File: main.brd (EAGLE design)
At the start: 130 x 65 mm, 302 parts, among them CN1 DC-012A-D010, CN2 JST GH 10 Pin, CN3 5.8ZSPT, CN4 8 PIN FFC, CN5 MC-118LS-H100, CN7 8 PIN FFC, Q1 GSFP0449, Q2 2SCR586D, Q3 MMBT3904, Q4 MMBT3906, Q5 MMBT3906, U1 TPS54302, U10 SN74LVC2G17, U11 SN74LVC2G17, U12 SN74LVC2G17, U13 SN74LVC2G17, U14 SN74LVC2G17, U15 SN74LVC2G17, U16 SN74LVC2G17, U17 SN74LVC2G17, U18 T8Q144C4, U19 SN74LVC2G17, U2 USBLC6-2SC6, U20 R2A20169SA#W5, U21 LM317MDT, U22 LM317MDT, U23 ADC101C027, U27 ADS7056, U28 AD5258BRMZ1-R7, U29 COS8092SR, U3 93LC56B-I/SN, U30 ADS7056, U31 AD5258BRMZ1-R7, U32 COS8092SR, U33 LM317MDT, U34 LM317MDT, U35 ADS7056, U36 AD5258BRMZ1-R7, U37 COS8092SR, U4 W25Q128JV, U41 ADS7056, U42 AD5258BRMZ1-R7, U43 COS8092SR, U44 ADS7056, U45 AD5258BRMZ1-R7, U46 COS8092SR, U5 TPS62065, U50 ADS7056, U51 AD5258BRMZ1-R7, U52 COS8092SR, U6 FT2232H, U7 TPS563201, U8 TCD2720BFG, U9 SN74LVC2G17

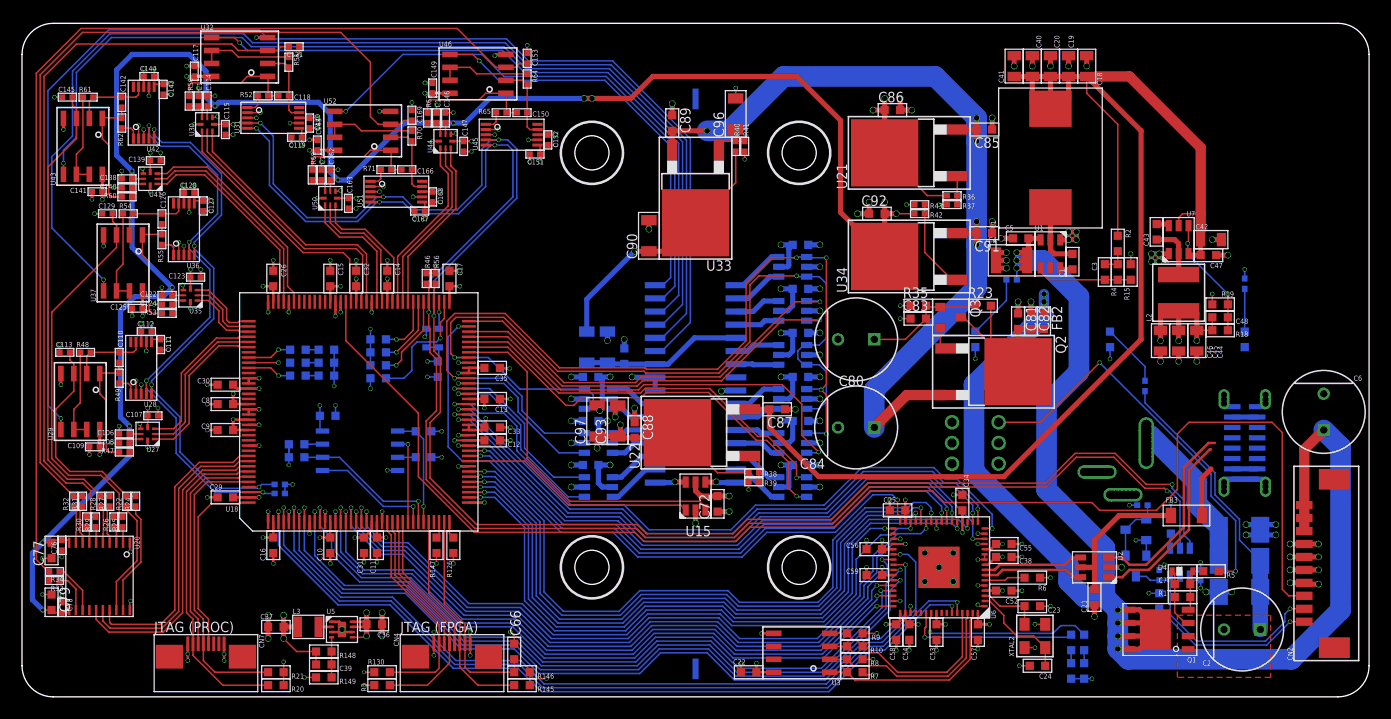
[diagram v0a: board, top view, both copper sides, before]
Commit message: Bits and pieces
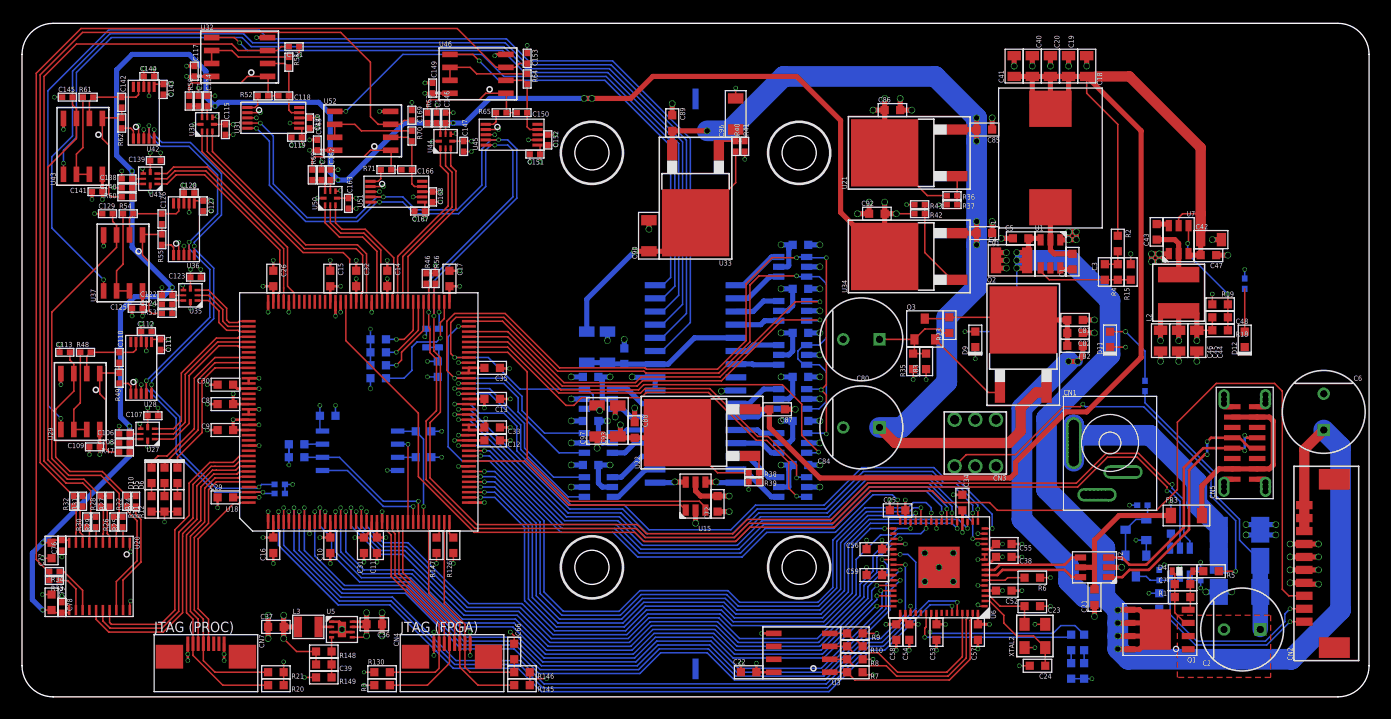
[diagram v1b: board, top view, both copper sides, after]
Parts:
- moved R59 22.5 mm to (-52.5, -13.9), flipped to the top, turned to 270 degrees
- moved R11 20.7 mm to (-51.2, -13.9), flipped to the top, turned to 270 degrees
- moved R12 19.0 mm to (-50.0, -13.9), flipped to the top, turned to 270 degrees
- moved D10 18.6 mm to (-52.5, -11.1), flipped to the top, turned to 270 degrees
- moved D5 16.9 mm to (-51.2, -11.1), flipped to the top, turned to 270 degrees
- moved D6 15.1 mm to (-50.0, -11.1), flipped to the top, turned to 270 degrees
- moved C81 5.50 mm to (36.6, 3.88), turned to 180 degrees
- moved R35 5.40 mm to (21.0, -0.12), turned to 90 degrees
- moved R58 4.53 mm to (31.0, 3.25), turned to 90 degrees
- moved C82 4.40 mm to (36.6, 2.62), turned to 180 degrees
- moved C83 4.19 mm to (22.2, -0.12), turned to 90 degrees
- moved Q2 3.95 mm to (31.6, 2.12), turned to 0 degrees
- moved FB2 3.83 mm to (36.6, 1.38), turned to 180 degrees
- moved R23 3.75 mm to (24.5, 3.38), turned to 90 degrees
- moved Q3 2.74 mm to (22.1, 3.00), turned to 0 degrees
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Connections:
- removed net PROC_STATUS: U18.117
- net LED_PROC_STATUS: now also U18.117
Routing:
- net LED_PROC_STATUS: track 0.00 -> 15.4 mm
- net PWR_ANA_UNREG: track 85.5 -> 98.4 mm
- net LED_PROC_SCANNING: track 4.31 -> 16.9 mm, vias 1 -> 0
- net N$5: track 14.9 -> 26.1 mm
- net LED_FPGA_STATUS: track 4.31 -> 14.4 mm, vias 1 -> 0
- net N$41: track 9.66 -> 18.9 mm
- net LED_PWM_CONT: track 133.1 -> 139.2 mm
- net N$13: track 18.4 -> 24.4 mm, vias 0 -> 2
- net N$40: track 2.43 -> 8.37 mm
- net N$12: track 18.8 -> 24.3 mm, vias 0 -> 2
- net PROC_STATUS: track 2.88 -> 0.00 mm, vias 1 -> 0
- net N$11: track 39.3 -> 42.0 mm
- net GND: track 251.0 -> 253.4 mm
- net N$39: track 11.9 -> 10.00 mm
- net PWR_SYS_12V: track 138.8 -> 140.5 mm
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
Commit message: New LED PCB formfactor. UART debug added to FPGA for softcore.
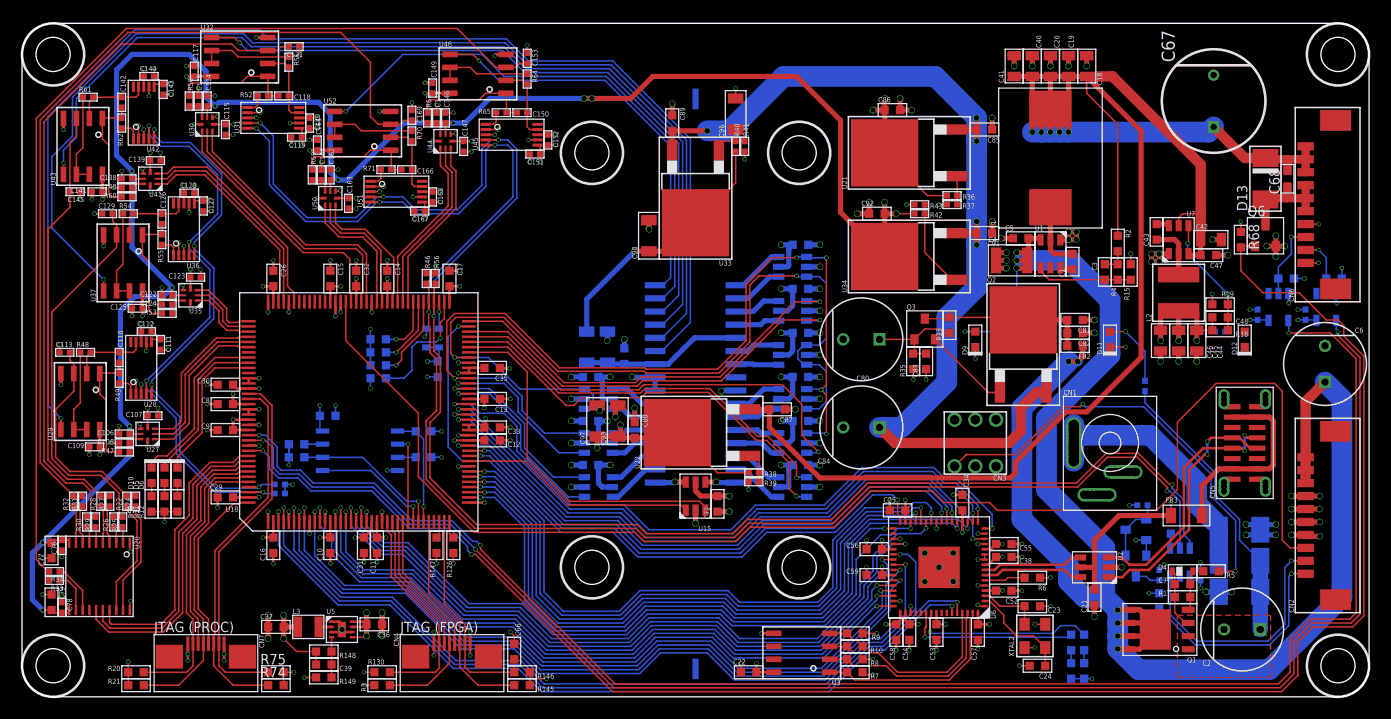
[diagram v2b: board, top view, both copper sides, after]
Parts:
- added C67: 470uF 25V, CAPACITORS:10MM_RADIAL_5MM_PITCH
- added C68: 0.1uF 50V, c_0603:0603
- added C69, C70: 0.1uF 16V, c_0402:0402
- added CN6: JST GH 10 Pin, CONNECTORs:1.25-10PWT
- added D13: B360A-13-F, DIODES:DO214AC
- added MECH5, MECH6, MECH7, MECH8: 6mm x 3mm, MISC:MOUNTHOLE_6X3
- added Q6: IRLML6244, TRANSISTORs:SOT23-3
- added R68, R72, R73, R74, R75: 10k, r_0603:0603
- added U24, U25: SCHMITT, ICs:SOT23-5
- moved R20 13.6 mm to (-54.0, -30.1), turned to 180 degrees
- moved R21 13.6 mm to (-54.0, -31.4), turned to 180 degrees
- moved C145 9.16 mm to (-59.9, 16.2), turned to 180 degrees
- moved R67 5.20 mm to (50.6, 2.75), turned to 0 degrees
- moved C6 4.63 mm to (60.8, -0.38)
- moved CN2 4.63 mm to (61.0, -15.0)
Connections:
- removed net N$76: U18.134
- removed net N$77: U18.132
- removed net N$78: U18.131
- removed net N$79: U18.124
- removed net N$80: U18.123
- new net MTR_PWM: Q6.1, R68.2, U18.134
- new net MTR_SENSE_A: U18.131, U24.4
- new net MTR_SENSE_B: U18.132, U25.4
- new net MTR_SENSE_IN_A: CN6.3, R72.2, U24.2
- new net MTR_SENSE_IN_B: CN6.2, R73.2, U25.2
- new net N$57: C68.1, CN6.5, CN6.6, CN6.7, D13.A, Q6.2
- new net PROC_UART_RX: CN7.2, R75.1, U18.123
- new net PROC_UART_TX: CN7.3, R74.1, U18.124
- net GND: now also C67.1, C69.1, C70.1, CN6.1, Q6.3, R68.1, R72.1, R73.1, U24.3, U25.3
- net PWR_SYS_12V: now also C67.2, C68.2, CN6.10, CN6.8, CN6.9, D13.K
- net PWR_SYS_3V3: now also C69.2, C70.2, CN6.4, R74.2, R75.2, U24.5, U25.5
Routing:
- net MTR_PWM: track 0.00 -> 167.6 mm, vias 0 -> 2
- net MTR_SENSE_A: track 0.00 -> 156.1 mm, vias 0 -> 3
- net MTR_SENSE_B: track 0.00 -> 152.4 mm, vias 0 -> 3
- net PWR_SYS_12V: track 140.5 -> 185.3 mm, vias 0 -> 5
- net PROC_UART_TX: track 0.00 -> 35.4 mm
- net PROC_UART_RX: track 0.00 -> 35.0 mm
- net GND: track 253.4 -> 264.7 mm, vias 251 -> 263
- net N$57: track 0.00 -> 10.3 mm
- net MTR_SENSE_IN_A: track 0.00 -> 7.34 mm, vias 0 -> 1
- net PWR_SYS_3V3: track 134.7 -> 140.9 mm, vias 66 -> 69
- net MTR_SENSE_IN_B: track 0.00 -> 5.76 mm, vias 0 -> 1
- net PWR_BUS_24V_UNREG: track 167.7 -> 172.6 mm
- net TEMP_SEN_B: track 16.4 -> 21.2 mm
- net TEMP_SEN_A: track 23.2 -> 28.0 mm
- net LED_PWM_CONT: track 139.2 -> 134.7 mm
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
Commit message: Cleared errors on PCB
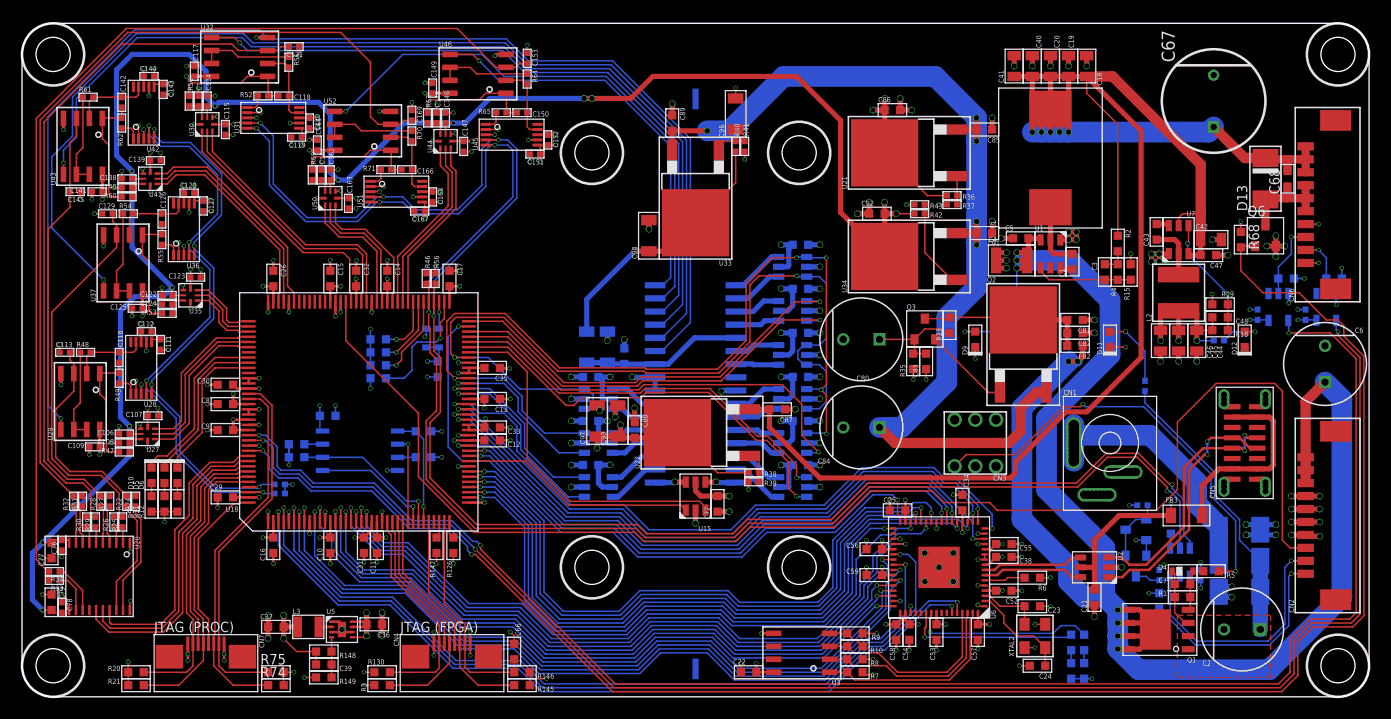
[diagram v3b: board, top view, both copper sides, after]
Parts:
- moved R67 0.88 mm to (50.5, 1.88)
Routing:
- net N$5: track 26.1 -> 31.4 mm
- net N$47: track 0.00 -> 4.36 mm, vias 0 -> 1
- net PWR_SYS_3V3: track 140.9 -> 142.6 mm
- net GND: track 264.7 -> 265.3 mm

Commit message: New formactor
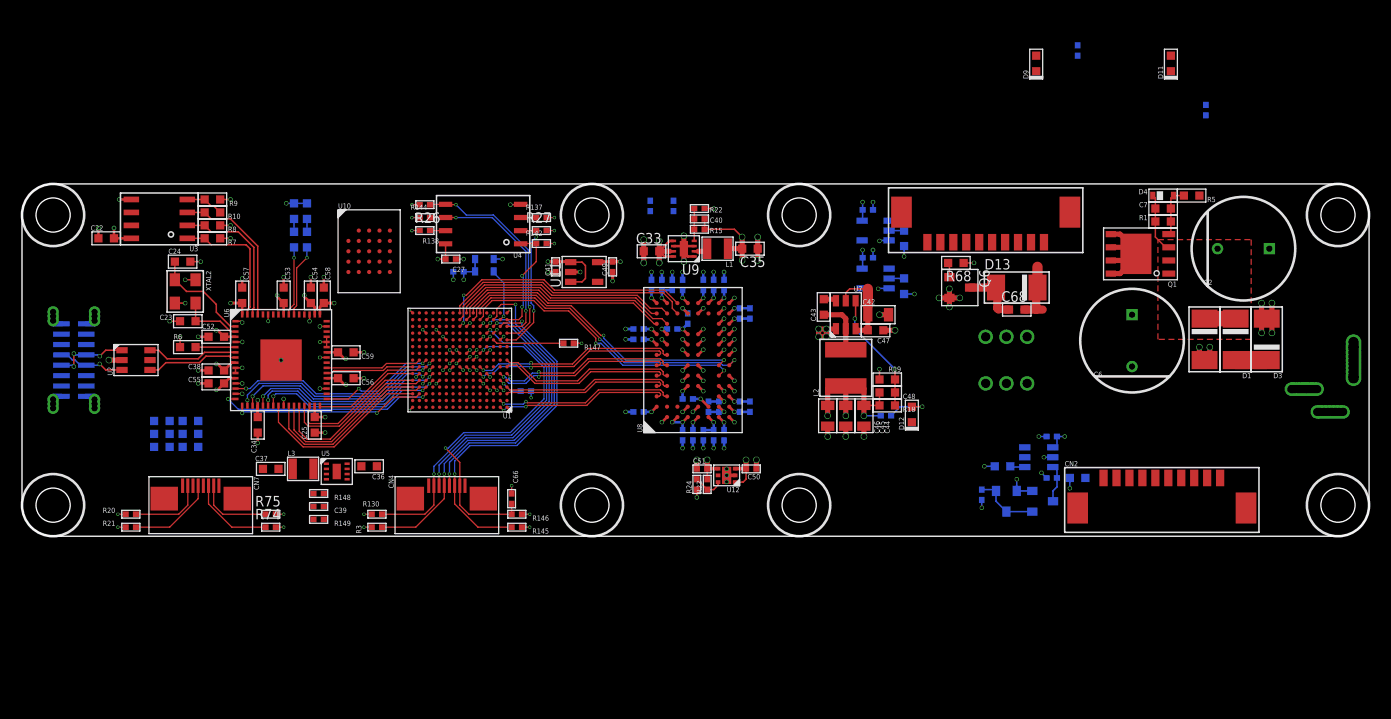
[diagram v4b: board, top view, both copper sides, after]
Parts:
- removed C106, C107, C109, C111, C112, C113, C114, C115, C117, C119, C120, C121, C122, C123, C125, C127, C128, C129, C138, C139, C141, C143, C144, C145, C146, C147, C149, C151, C152, C153, C162, C163, C165, C167, C168, C169, C76, C78: 0.1uF 16V, c_0402:0402
- removed C108, C116, C124, C140, C148, C164: 220pF 25V, c_0402:0402
- removed C110, C118, C126, C142, C150, C166: NO FIT, c_0402:0402
- removed C61, C62, C63, C71, C72, C73, C74, C75: 100nF 16V, CAPACITORS:0603
- removed C67: 470uF 25V, CAPACITORS:10MM_RADIAL_5MM_PITCH
- removed C77, C79: 10uF 10V, c_0603:0603
- removed C80, C84: 100uF 50V, CAPACITORS:8MM_RADIAL_3.5MM_PITCH
- removed C81, C83, C85, C87, C89, C91: 0.1uF 50V, c_0603:0603
- removed C82: 100pF 50V, c_0603:0603
- removed C86, C88, C92: 1uF 10V, c_0603:0603
- removed C90: 1uF 16V, c_1206:1206
- removed C93, C96, C97: 10uF 10V, c_1206:1206
- removed FB1, FB3: 150R 100MHz, INDUCTORS:1206
- removed FB2: 600R, INDUCTORS:0603
- removed Q2: 2SCR586D, TRANSISTORs:TO252
- removed Q3: MMBT3904, TRANSISTORs:SOT23-3
- removed R126, R139, R140, R141: 10k, r_0603:0603
- removed R25, R29, R31, R33: 430R, r_0402:0402
- removed R28, R30, R32, R34: 110k, r_0402:0402
- removed R35: 20k, r_0603:0603
- removed R36, R38, R40, R42: 240R, r_0402:0402
- removed R37, R39: 715R, r_0402:0402
- removed R41: 1.69k, r_0402:0402
- removed R43: 390R, r_0402:0402
- removed R44, R45, R46, R56: 2.2k, r_0402:0402
- removed R47, R50, R53, R60, R63, R69: 100R, r_0402:0402
- removed R48, R51, R54, R61, R64, R70: 330R, r_0402:0402
- removed R49, R52, R55, R62, R65, R71: 680R, r_0402:0402
- removed U13, U14, U15, U16, U17, U19: SN74LVC2G17, ICs:SOT23-6
- removed U18: T8Q144C4, ICs:QFP144
- removed U20: R2A20169SA#W5, ICs:TSSOP20
- removed U21, U22, U33, U34: LM317MDT, ICs:TO252-2
- removed U27, U30, U35, U41, U44, U50: ADS7056, ICs:X2QFN8
- removed U28, U31, U36, U42, U45, U51: AD5258BRMZ1-R7, ICs:MSOP10
- removed U29, U32, U37, U43, U46, U52: COS8092SR, ICs:SO8
- C1, C51: value 100nF 16V -> 1uF 10V; device CAPACITORS:0603 -> c_0402:0402
- C10, C14, C17, C29, C31: value 100nF 16V -> 10uF 6.3V; device CAPACITORS:0603 -> c_0402:0402
- C11, C12, C13, C15, C16, C26, C27, C28, C30, C32, C60, C66, C8, C9: value 100nF 16V -> 0.1uF 16V; device CAPACITORS:0603 -> c_0402:0402
- C18, C19, C20: value 10uF 50V -> 0.1uF 16V; device CAPACITORS:0805 -> c_0402:0402
- C2, C6: value 100uF 50V -> 470uF 25V; device CAPACITORS:8MM_RADIAL_3.5MM_PITCH -> CAPACITORS:10MM_RADIAL_5MM_PITCH
- C21: device c_0603:0603 -> c_0402:0402
- C3: value 100pF 50V -> 10uF 6.3V; device c_0603:0603 -> c_0402:0402
- C33, C35: value 100nF 16V -> 10uF 6.3V; device CAPACITORS:0603 -> c_0603:0603
- C39: value 33pF 10V -> 150pF 25V; device c_0603:0603 -> c_0402:0402
- C4: value 10uF 50V -> 0.1uF 16V; device CAPACITORS:1210 -> c_0402:0402
- C40: value 10uF 50V -> 150pF 25V; device CAPACITORS:0805 -> c_0402:0402
- C41: value 10uF 50V -> 1uF 10V; device CAPACITORS:0805 -> c_0402:0402
- C49: value 100nF 16V -> 2.2uF 6.3V; device CAPACITORS:0603 -> c_0402:0402
- C5: value 0.1uF 50V -> 0.1uF 16V; device c_0603:0603 -> c_0402:0402
- C50: value 10uF 25V -> 1uF 10V; device c_1206:1206 -> c_0402:0402
- L1: value 15uH 6.5A -> 1uH; device INDUCTORS:SRP1035A -> INDUCTORS:1008
- R130, R137, R138, R142, R143, R144, R145, R146, R147, R20, R21, R3, R74, R75: device r_0603:0603 -> r_0402:0402
- R148: value 180k -> 36k; device r_0603:0603 -> r_0402:0402
- R149: value 180k -> 62k; device r_0603:0603 -> r_0402:0402
- R15: value 5.23k -> 36k; device r_0603:0603 -> r_0402:0402
- R2: value 51k -> 1.5k; device RESISTORS:0603 -> r_0402:0402
- R22: value 430R -> 62k
- R23: value 10k -> 30k; device r_0603:0603 -> r_0402:0402
- R24: value 110k -> 12k
- R26: value 110k -> 10k
- R27: value 430R -> 10k
- R4: value 100k -> 1.5k; device r_0603:0603 -> r_0402:0402
- U1: value TPS54302 -> Ti60F225C4; device ICs:SOT23-6 -> ICs:FBGA225
- U10: value SN74LVC2G17 -> W958D8NBYA5I; device ICs:SOT23-6 -> ICs:VBGA24
- U11: value SN74LVC2G17 -> TPS70918; device ICs:SOT23-6 -> ICs:SOT23-5
- U12: value SN74LVC2G17 -> AP7335; device ICs:SOT23-6 -> ICs:DFN2020-6
- U8: value TCD2720BFG -> AR0822; device ICs:WQFN32-C-R300-1.27 -> ICs:PBGA75
- U9: value SN74LVC2G17 -> TPS62065; device ICs:SOT23-6 -> ICs:WSON8
- moved CN5 113.3 mm to (-60.0, 0.00), flipped to the bottom
- moved U2 94.6 mm to (-54.0, 0.00), turned to 90 degrees
- moved C24 91.3 mm to (-49.5, 9.50), turned to 180 degrees
- moved XTAL2 88.5 mm to (-49.2, 6.62), turned to 270 degrees
- moved R13 88.2 mm to (-38.8, 14.4), turned to 90 degrees
- moved R14 86.1 mm to (-37.5, 14.4), turned to 90 degrees
- moved C23 86.0 mm to (-49.0, 3.75), turned to 0 degrees
- moved D7 85.6 mm to (-38.8, 11.6), turned to 90 degrees
- moved R6 84.5 mm to (-49.0, 1.25), turned to 0 degrees
- moved D8 83.4 mm to (-37.5, 11.6), turned to 90 degrees
- moved C52 79.9 mm to (-46.2, 2.25), turned to 0 degrees
- moved C38 78.1 mm to (-46.2, -1.00), turned to 0 degrees
- moved C57 78.1 mm to (-43.8, 6.25), turned to 270 degrees
- moved C55 77.6 mm to (-46.2, -2.25), turned to 0 degrees
- moved C22 74.8 mm to (-56.9, 11.8)
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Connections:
- removed net ADC_SPI_MISO_1: U18.113, U27.2
- removed net ADC_SPI_MISO_2: U18.110, U35.2
- removed net ADC_SPI_MISO_3: U18.105, U41.2
- removed net ADC_SPI_MISO_4: U18.90, U30.2
- removed net ADC_SPI_MISO_5: U18.82, U44.2
- removed net ADC_SPI_MISO_6: U18.86, U50.2
- removed net ADC_SPI_NCS_1: U18.114, U27.1
- removed net ADC_SPI_NCS_2: U18.111, U35.1
- removed net ADC_SPI_NCS_3: U18.106, U41.1
- removed net ADC_SPI_NCS_4: U18.92, U30.1
- removed net ADC_SPI_NCS_5: U18.83, U44.1
- removed net ADC_SPI_NCS_6: U18.87, U50.1
- removed net ADC_SPI_SCLK_1: U18.112, U27.3
- removed net ADC_SPI_SCLK_2: U18.109, U35.3
- removed net ADC_SPI_SCLK_3: U18.103, U41.3
- removed net ADC_SPI_SCLK_4: U18.89, U30.3
- removed net ADC_SPI_SCLK_5: U18.81, U44.3
- removed net ADC_SPI_SCLK_6: U18.84, U50.3
- removed net CCD_1A1: U8.1, U9.6
- removed net CCD_1A2: U8.8
- removed net CCD_1A3: U11.6, U8.10
- removed net CCD_1A4: U12.6, U8.12
- removed net CCD_1A5: U17.4, U8.21
- removed net CCD_2A1: U8.2, U9.4
- removed net CCD_2A2: U10.4, U8.7
- removed net CCD_2A3: U11.4, U8.11
- removed net CCD_2A4: U19.6, U8.22
- removed net CCD_2A5: U19.4, U8.23
- removed net CCD_2B: U10.6, U8.6
- removed net CCD_CP: U13.6, U8.3
- removed net CCD_RS: U13.4, U8.4
- removed net CCD_SH_M1: U15.4, U8.16
- removed net CCD_SH_M2: U15.6, U8.17
- removed net CCD_SH_S1: U14.4, U8.15
- removed net CCD_SH_S2: U16.6, U8.18
- removed net CCD_SH_S3: U14.6, U8.14
- removed net CCD_SH_S4: U16.4, U8.19
- removed net CCD_SIG_1A: U11.1, U12.1, U17.3, U18.61, U9.1
- removed net CCD_SIG_2A: U10.1, U10.3, U11.3, U18.65, U19.1, U19.3, U9.3
- removed net CCD_SIG_CP: U13.1, U18.72
- removed net CCD_SIG_RS: U13.3, U18.70
- removed net CCD_SIG_SH_M1: U15.3, U18.66
- removed net CCD_SIG_SH_M2: U15.1, U18.45
- removed net CCD_SIG_SH_S1: U14.3, U18.67
- removed net CCD_SIG_SH_S2: U16.1, U18.58
- removed net CCD_SIG_SH_S3: U14.1, U18.68
- removed net CCD_SIG_SH_S4: U16.3, U18.59
- removed net CCD_SIG_SW: U17.1, U18.60
- removed net CCD_SIG_TG: U12.3, U18.69
- removed net CCD_SW: U17.6, U8.20
- removed net CCD_TG: U12.4, U8.13
- removed net DAC_SPI_MOSI: U18.135, U20.17
- removed net DAC_SPI_NCS: U18.137, U20.15
- removed net DAC_SPI_SCLK: U18.136, U20.16
- removed net FPGA_CONF_CBUS_0: R141.1, U18.78
- removed net FPGA_CONF_CBUS_1: R140.1, U18.79
- removed net FPGA_CONF_CBUS_2: R139.1, U18.80
- removed net FT_CONT_NCTS: U18.10, U6.41
- removed net FT_CONT_NDCD: U18.11, U6.45
- removed net FT_CONT_NDSR: U18.16, U6.44
- removed net FT_CONT_NDTR: U18.8, U6.43
- removed net FT_CONT_NRI: U18.15, U6.46
- removed net FT_CONT_NRTS: U18.7, U6.40
- removed net FT_CONT_PWRSAV: U18.3, U6.59
- removed net FT_CONT_TXDEN: U18.14, U6.48
- removed net FT_NPWREN: U18.4, U6.60
- removed net FT_NSUSPEND: U18.18, U6.36
- removed net MTR_PWM: Q6.1, R68.2, U18.134
- removed net N$100: R70.1, U52.6, U52.7
- removed net N$101: U18.100
- removed net N$102: U18.99
- removed net N$103: U18.98
- removed net N$104: U18.97
- removed net N$145: R126.2, U18.36
- removed net N$21: C49.2, C50.2, FB1.2, U8.26, U8.5
- removed net N$22: R22.1, U20.18
- removed net N$23: R24.1, U20.19
- removed net N$26: R25.1, U20.2
- removed net N$27: R26.1, U20.3
- removed net N$28: R27.1, U20.4
- removed net N$29: R28.1, U20.5
- removed net N$30: R29.1, U20.6
- removed net N$31: R30.1, U20.7
- removed net N$32: R31.1, U20.8
- removed net N$33: R32.1, U20.9
- removed net N$34: R33.1, U20.12
- removed net N$35: R34.1, U20.13
- removed net N$36: C81.2, C82.2, FB2.2, Q2.2, Q3.2, R23.2
- removed net N$39: C80.P, C83.2, Q3.1, R23.1, R35.2
- removed net N$40: Q2.1, Q3.3
- removed net N$41: CN5.A4, CN5.A9, CN5.B4, CN5.B9, FB3.1
- removed net N$52: R36.1, R37.2, U21.1
- removed net N$53: R38.1, R39.2, U22.1
- removed net N$54: C96.2, R40.1, R41.2, U33.1
- removed net N$55: R42.1, R43.2, U34.1
- removed net N$59: U18.102
- removed net N$60: U18.101
- removed net N$61: C108.2, R47.2, U27.7
- removed net N$62: C110.2, R47.1, R49.2, U29.1
- removed net N$63: C110.1, R48.2, U28.9, U29.2
- removed net N$64: R49.1, U28.1
- removed net N$65: R48.1, U29.6, U29.7
- removed net N$66: C116.2, R50.2, U30.7
- removed net N$67: C118.2, R50.1, R52.2, U32.1
- removed net N$68: C118.1, R51.2, U31.9, U32.2
- removed net N$69: R52.1, U31.1
- removed net N$70: R51.1, U32.6, U32.7
- removed net N$71: C124.2, R53.2, U35.7
- removed net N$72: C126.2, R53.1, R55.2, U37.1
- removed net N$73: C126.1, R54.2, U36.9, U37.2
- removed net N$74: R55.1, U36.1
- removed net N$75: R54.1, U37.6, U37.7
- removed net N$81: C140.2, R60.2, U41.7
- removed net N$82: C142.2, R60.1, R62.2, U43.1
- removed net N$83: C142.1, R61.2, U42.9, U43.2
- removed net N$84: R62.1, U42.1
- removed net N$85: R61.1, U43.6, U43.7
- removed net N$86: C148.2, R63.2, U44.7
- removed net N$87: C150.2, R63.1, R65.2, U46.1
- removed net N$88: C150.1, R64.2, U45.9, U46.2
- removed net N$89: R65.1, U45.1
- removed net N$9: C3.1, R15.2, R4.1, U1.4
- removed net N$90: R64.1, U46.6, U46.7
- removed net N$91: U18.119
- removed net N$95: U18.115
- removed net N$96: C164.2, R69.2, U50.7
- removed net N$97: C166.2, R69.1, R71.2, U52.1
- removed net N$98: C166.1, R70.2, U51.9, U52.2
- removed net N$99: R71.1, U51.1
- removed net POT_I2C0_SCL: R44.1, U18.141, U28.5, U36.5, U42.5
- removed net POT_I2C0_SDA: R45.1, U18.142, U28.4, U36.4, U42.4
- removed net PWR_ANA_10V: C90.2, FB1.1, R40.2, U33.2
- removed net PWR_ANA_3V3: C106.2, C114.2, C122.2, C138.2, C146.2, C162.2, C76.2, C77.2, C78.2, C79.2, C92.2, R42.2, U20.10, U20.11, U27.6, U30.6, U34.2, U35.6, U41.6, U44.6, U50.6
- removed net PWR_ANA_5V: C109.2, C112.2, C117.2, C120.2, C125.2, C128.2, C141.2, C144.2, C149.2, C152.2, C165.2, C168.2, C86.2, R36.2, U21.2, U28.8, U29.8, U31.8, U32.8, U36.8, U37.8, U42.8, U43.8, U45.8, U46.8, U51.8, U52.8
- removed net PWR_ANA_UNREG: C84.P, C85.2, C89.2, C91.2, Q2.3, U21.3, U33.3, U34.3
- removed net PWR_BUS_24V_UNREG: C4.2, C5.2, C6.P, CN2.10, CN2.8, CN2.9, FB2.1, Q1.5, Q1.6, Q1.7, Q1.8, Q1.PAD, R58.2, U1.3
- removed net PWR_CLK_5V: C51.2, C60.2, C61.2, C62.2, C63.2, C71.2, C72.2, C73.2, C74.2, C75.2, C88.2, C93.2, C97.2, R38.2, U10.5, U11.5, U12.5, U13.5, U14.5, U15.5, U16.5, U17.5, U19.5, U22.2, U9.5
- removed net PWR_FPGA_1V2: C10.2, C11.2, C12.2, C13.2, C14.2, C15.2, C16.2, C17.2, C26.2, C37.2, C39.2, C8.2, C9.2, L3.2, R148.2, U18.107, U18.125, U18.128, U18.13, U18.130, U18.2, U18.22, U18.49, U18.57, U18.73, U18.85, U18.96
- removed net PWR_SYS_12V: C18.2, C19.2, C20.2, C40.2, C41.2, C42.2, C47.2, C67.2, C68.2, C87.2, CN6.10, CN6.8, CN6.9, D13.K, L1.2, R2.2, U22.3, U7.3, U7.5
- removed net PWR_USB_VBUS: C21.2, FB3.2, U2.5
- removed net SEN_OFFSET_OS1: C113.2, R22.2, R24.2, U29.3
- removed net SEN_OFFSET_OS2: C129.2, R25.2, R26.2, U37.3
- removed net SEN_OFFSET_OS3: C145.2, R27.2, R28.2, U43.3
- removed net SEN_OFFSET_OS4: C121.2, R29.2, R30.2, U32.3
- removed net SEN_OFFSET_OS5: C153.2, R33.2, R34.2, U46.3
- removed net SEN_OFFSET_OS6: C169.2, R31.2, R32.2, U52.3
- removed net SEN_SIG_OS1: U29.5, U8.27
- removed net SEN_SIG_OS2: U37.5, U8.28
- removed net SEN_SIG_OS3: U43.5, U8.29
- removed net SEN_SIG_OS4: U32.5, U8.30
- removed net SEN_SIG_OS5: U46.5, U8.32
- removed net SEN_SIG_OS6: U52.5, U8.31
- new net AR_CLK: U1.P6, U8.G6
- new net AR_GPIO0: U1.P7, U8.B10
- new net AR_GPIO1: U1.R6, U8.A10
- new net AR_GPIO2: U1.P8, U8.B11
- new net AR_GPIO3: U1.R7, U8.A11
- new net AR_I2C_SCL: R4.1, U1.R8, U8.C11
- new net AR_I2C_SDA: R2.1, U1.N8, U8.C12
- new net AR_MIPI_CLK_N: U1.G1, U8.A5
- new net AR_MIPI_CLK_P: U1.H1, U8.B5
- new net AR_MIPI_D0_N: U1.F5, U8.A7
- new net AR_MIPI_D0_P: U1.G5, U8.B7
- new net AR_MIPI_D1_N: U1.F2, U8.A6
- new net AR_MIPI_D1_P: U1.F1, U8.B6
- new net AR_MIPI_D2_N: U1.C1, U8.A4
- new net AR_MIPI_D2_P: U1.D1, U8.B4
- new net AR_MIPI_D3_N: U1.A2, U8.A3
- new net AR_MIPI_D3_P: U1.B2, U8.B3
- new net AR_NRESET: U1.R5, U8.H6
- new net AR_XSHUTDOWN: U1.P5, U8.G5
- new net MTR_CONT_PWM: Q6.1, R68.2
- new net N$19: R23.1, R24.2, U12.6
- new net PWR_BUS_UNREG: C42.2, C47.2, C6.2, C68.2, CN2.10, CN2.8, CN2.9, CN6.1, CN6.2, CN6.3, D13.K, Q1.5, Q1.6, Q1.7, Q1.8, Q1.PAD, R58.2, U7.3, U7.5
- new net PWR_FPGA_0V95: C37.2, C39.2, L3.2, R148.2, U1.E13, U1.E5, U1.G10, U1.G7, U1.G9, U1.H6, U1.H8, U1.J7, U1.J9, U1.L10, U1.L5, U1.M3
- new net PWR_FPGA_1V8: U1.D4, U1.E11, U1.L4, U1.M11
- new net PWR_MIPI_1V2: R143.2, U1.D2, U1.F4
- new net PWR_SEN_1V05D: C17.2, C18.2, C19.2, C20.2, C21.2, C26.2, C29.2, C30.2, C31.2, C32.2, C35.2, C40.2, L1.2, R15.2, U8.A12, U8.A8, U8.A9, U8.B8, U8.D12, U8.E12, U8.F1, U8.G12, U8.G2
- new net PWR_SEN_2V8A: C10.2, C11.2, C12.2, C13.2, C14.2, C15.2, C16.2, C51.2, C60.2, R23.2, U12.4, U8.A2, U8.C1, U8.D1, U8.F12, U8.G1, U8.H11, U8.H12, U8.H2
- new net PWR_SYS_1V8: C3.2, C4.2, C49.2, C5.2, C8.2, C9.2, R2.2, R4.2, U1.N5, U1.N7, U11.5, U8.B12, U8.B9, U8.D11, U8.E1
- net FLS_SPI_CLK: now also U1.N1; no longer U18.30
- net FLS_SPI_MISO: now also R27.1, U1.L1; no longer U18.28
- net FLS_SPI_MOSI: now also R26.1, U1.M1; no longer U18.29
- net FLS_SPI_NCS: now also U1.P1; no longer U18.31
- net FPGA_CLK_33M: now also U1.P2; no longer U18.75
- net FPGA_CONF_CDONE: now also U1.L3; no longer U18.34
- net FPGA_CONF_CSI: now also U1.N2; no longer U18.32
- net FPGA_CONF_NCRST: now also U1.J5; no longer U18.35
- net FPGA_CONF_NTEST: now also U1.E2; no longer U18.74
- net FPGA_JTAG_TCK: now also U1.N4; no longer U18.26
- net FPGA_JTAG_TDI: now also U1.P3; no longer U18.27
- net FPGA_JTAG_TDO: now also U1.M4; no longer U18.24
- net FPGA_JTAG_TMS: now also U1.N3; no longer U18.25
- net FT_CLKOUT: now also U1.G14; no longer U18.71
- net FT_CONT_RX: now also U1.H14; no longer U18.17
- net FT_CONT_TX: now also U1.G15; no longer U18.6
- net FT_D0: now also U1.C13; no longer U18.56
- net FT_D1: now also U1.C14; no longer U18.55
- net FT_D2: now also U1.G13; no longer U18.54
- net FT_D3: now also U1.F13; no longer U18.40
- net FT_D4: now also U1.F12; no longer U18.39
- net FT_D5: now also U1.E12; no longer U18.48
- net FT_D6: now also U1.D13; no longer U18.47
- net FT_D7: now also U1.C15; no longer U18.46
- net FT_NOE: now also U1.H13; no longer U18.38
- net FT_NRD: now also U1.E14; no longer U18.42
- net FT_NRST: now also U1.H12; no longer U18.53
- net FT_NRXF: now also U1.D14; no longer U18.43
- net FT_NSIWU: now also U1.F15; no longer U18.20
- net FT_NTXE: now also U1.D15; no longer U18.19
- net FT_NWR: now also U1.E15; no longer U18.41
- net GND: now also C1.1, C2.1, C3.1, C6.1, CN6.10, R22.1, R24.1, U1.A1, U1.A15, U1.D3, U1.G6, U1.G8, U1.H7, U1.H9, U1.J6, U1.J8, U1.M13, U1.R1, U1.R15, U10.B3, U10.C1, U10.E5, U12.7, U6.41, U6.43, U6.44, U6.45, U8.B1, U8.D2, U8.D4, U8.D5, U8.D6, U8.D7, U8.D8, U8.D9, U8.E11, U8.E2, U8.E4, U8.E5, U8.E6, U8.E7, U8.E8, U8.E9, U8.G10, U8.G11, U8.G3, U8.G4, U8.G7, U8.G8, U8.G9, U8.H1, U8.H10, U8.H3, U8.H4, U8.H5, U8.H7, U8.H8, U8.H9, U9.1, U9.3, U9.6, U9.PAD; no longer C106.1, C107.1, C108.1, C109.1, C111.1, C112.1, C113.1, C114.1, C115.1, C116.1, C117.1, C119.1, C120.1, C121.1, C122.1, C123.1, C124.1, C125.1, C127.1, C128.1, C129.1, C138.1, C139.1, C140.1, C141.1, C143.1, C144.1, C145.1, C146.1, C147.1, C148.1, C149.1, C151.1, C152.1, C153.1, C162.1, C163.1, C164.1, C165.1, C167.1, C168.1, C169.1, C2.N, C40.1, C6.N, C61.1, C62.1, C63.1, C67.1, C71.1, C72.1, C73.1, C74.1, C75.1, C76.1, C77.1, C78.1, C79.1, C80.N, C81.1, C82.1, C83.1, C84.N, C85.1, C86.1, C87.1, C88.1, C89.1, C90.1, C91.1, C92.1, C93.1, C96.1, C97.1, CN6.1, R126.1, R15.1, R35.1, R37.1, R39.1, R41.1, R43.1, U1.1, U10.2, U13.2, U14.2, U15.2, U16.2, U17.2, U18.1, U18.104, U18.108, U18.120, U18.121, U18.126, U18.127, U18.129, U18.133, U18.37, U18.44, U18.5, U18.50, U18.64, U18.9, U18.94, U19.2, U20.1, U20.20, U27.5, U27.8, U28.2, U28.3, U28.7, U29.4, U30.5, U30.8, U31.2, U31.3, U31.7, U32.4, U35.5, U35.8, U36.3, U36.7, U37.4, U41.5, U41.8, U42.2, U42.7, U43.4, U44.5, U44.8, U45.3, U45.7, U46.4, U50.5, U50.8, U51.2, U51.7, U52.4, U8.24, U8.25, U8.9, U9.2
- net LED_FPGA_STATUS: no longer U18.118
- net LED_PROC_SCANNING: no longer U18.116
- net LED_PROC_STATUS: no longer U18.117
- net LED_PWM_CONT: no longer U18.93
- net MTR_SENSE_A: no longer U18.131
- net MTR_SENSE_B: no longer U18.132
- net MTR_SENSE_IN_A: now also CN6.8; no longer CN6.3
- net MTR_SENSE_IN_B: now also CN6.9; no longer CN6.2
- net N$2: now also L1.1, U9.2; no longer C1.1, U1.6
- net N$57: now also CN6.4; no longer CN6.7
- net N$6: now also U8.F2; no longer L1.1, U1.2
- net N$7: now also C40.1, R15.1, R22.2, U9.4; no longer C3.2, R2.1, R4.2
- net POT_I2C1_SCL: no longer R46.1, U18.77, U31.5, U45.5, U51.5
- net POT_I2C1_SDA: no longer R56.1, U18.76, U31.4, U45.4, U51.4
- net PROC_JTAG_TCK: no longer U18.140
- net PROC_JTAG_TDI: no longer U18.144
- net PROC_JTAG_TDO: no longer U18.138
- net PROC_JTAG_TMS: no longer U18.139
- net PROC_UART_RX: no longer U18.123
- net PROC_UART_TX: no longer U18.124
- net PWR_SYS_3V3: now also C41.2, C50.2, CN6.7, R26.2, R27.2, U1.F14, U1.G12, U1.J4, U1.L2, U1.P4, U11.1, U11.3, U12.1, U12.3, U6.59, U9.5, U9.7, U9.8; no longer C107.2, C111.2, C115.2, C119.2, C123.2, C127.2, C139.2, C143.2, C147.2, C151.2, C163.2, C167.2, C29.2, C30.2, C31.2, C32.2, C35.2, CN6.4, R139.2, R140.2, R141.2, R143.2, R44.2, R45.2, R46.2, R56.2, U18.12, U18.122, U18.143, U18.21, U18.23, U18.51, U18.52, U18.62, U18.63, U18.88, U18.91, U18.95, U27.4, U28.6, U30.4, U31.6, U35.4, U36.2, U36.6, U41.4, U42.3, U42.6, U44.4, U45.2, U45.6, U50.4, U51.3, U51.6
- net PWR_SYS_VIN: now also C2.2; no longer C2.P
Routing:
- net PWR_ANA_3V3: track 188.8 -> 0.00 mm, vias 12 -> 0
- net PWR_SYS_12V: track 185.1 -> 0.00 mm, vias 5 -> 0
- net PWR_BUS_24V_UNREG: track 172.6 -> 0.00 mm, vias 9 -> 0
- net MTR_PWM: track 167.6 -> 0.00 mm, vias 2 -> 0
- net PWR_FPGA_1V2: track 166.4 -> 0.00 mm, vias 13 -> 0
- net POT_I2C1_SDA: track 165.6 -> 0.00 mm, vias 5 -> 0
- net POT_I2C1_SCL: track 163.3 -> 0.00 mm, vias 5 -> 0
- net MTR_SENSE_A: track 156.1 -> 0.00 mm, vias 3 -> 0
- net MTR_SENSE_B: track 152.4 -> 0.00 mm, vias 3 -> 0
- net LED_PWM_CONT: track 134.7 -> 0.00 mm
- net GND: track 265.3 -> 134.3 mm, vias 263 -> 142
- net SEN_SIG_OS1: track 122.8 -> 0.00 mm, vias 1 -> 0
- net SEN_SIG_OS2: track 108.4 -> 0.00 mm, vias 1 -> 0
- net PWR_ANA_UNREG: track 98.4 -> 0.00 mm, vias 5 -> 0
- net SEN_OFFSET_OS5: track 97.8 -> 0.00 mm
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- added copper zone on layer 3, net PWR_SEN_1V05D
- added copper zone on layer 3, net PWR_SEN_2V8A
- removed copper zone on layer 3, net PWR_ANA_5V
- removed copper zone on layer 3, net PWR_CLK_5V
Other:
- board size 130 x 65 mm -> 130 x 34 mm
- board text removed: "JTAG (FPGA)"
- board text removed: "JTAG (PROC)"
